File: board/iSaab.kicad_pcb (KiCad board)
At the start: 2 copper layers, 58.5 x 65.1 mm, 29 parts, among them IC1 MCP2515, IC2 HVD251, IC3 MEGA328, IC4 7805

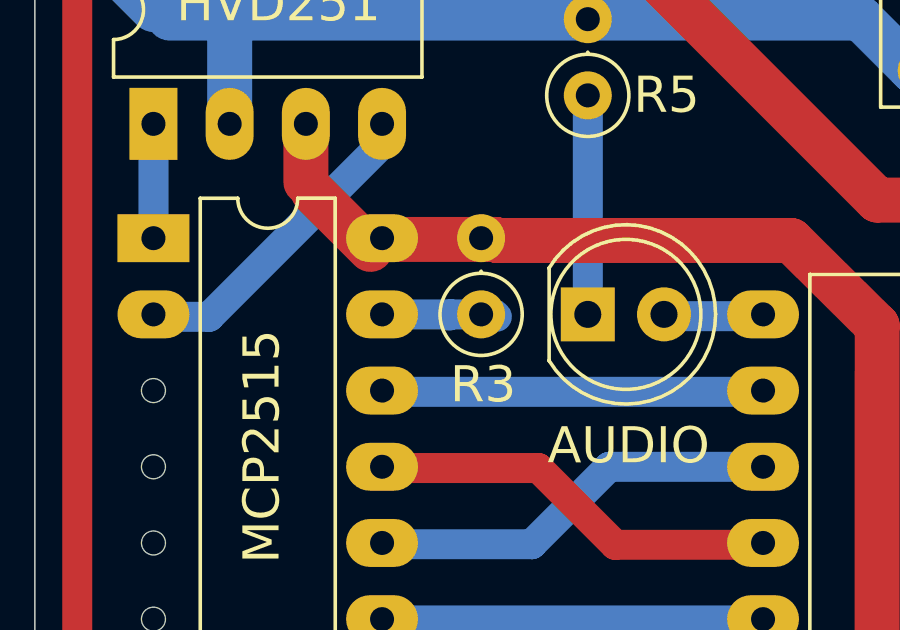
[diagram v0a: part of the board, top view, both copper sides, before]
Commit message: net clean-up
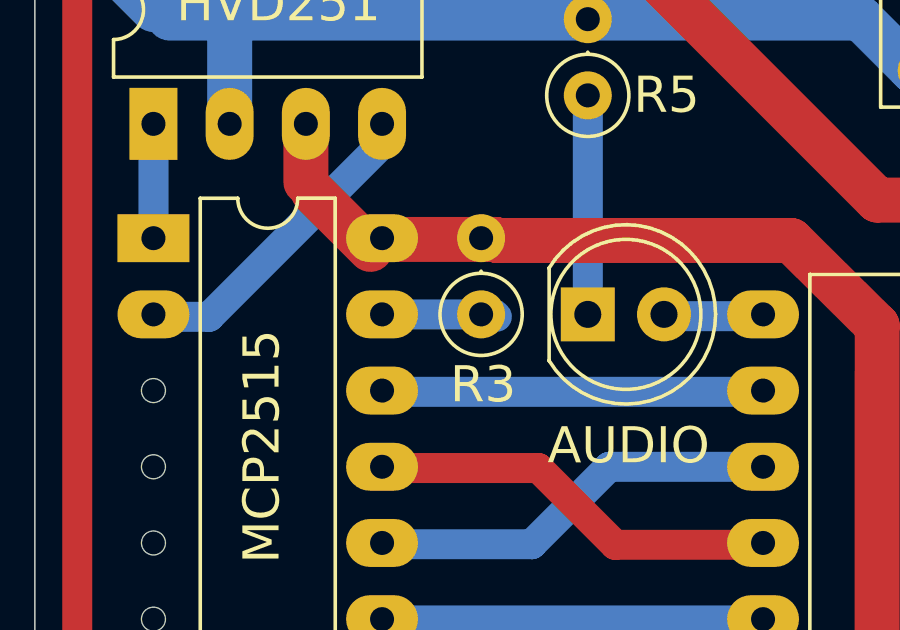
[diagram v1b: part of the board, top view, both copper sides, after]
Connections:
- net N$1 renamed TXCAN
- net N$10 renamed STDBY
- net N$12 renamed INT
- net N$14 renamed RESET
- net N$16 renamed XRESET
- net N$2 renamed RXCAN
- net N$31 renamed RX1BF
- net N$4 renamed OSC1
- net N$5 renamed OSC2
- net N$6 renamed TOSC2
- net N$7 renamed TOSC1
- Audio In pad 1: (no net) -> N$17
- Audio In pad 3: (no net) -> N$18
- IC1 pad 11: N$18 -> RX0BF
- R4 pad 2: N$18 -> RX0BF
- R6 pad 2: (no net) -> N$17
- R7 pad 2: (no net) -> N$18
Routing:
- net (no net): track 6.62 -> 0.00 mm
- net RX0BF: track 0.00 -> 5.15 mm
- net N$17: track 0.00 -> 3.62 mm
- net N$18: track 5.15 -> 3.00 mm
